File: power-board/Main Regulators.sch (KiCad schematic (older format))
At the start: 19 parts, among them U201 LMZ23610

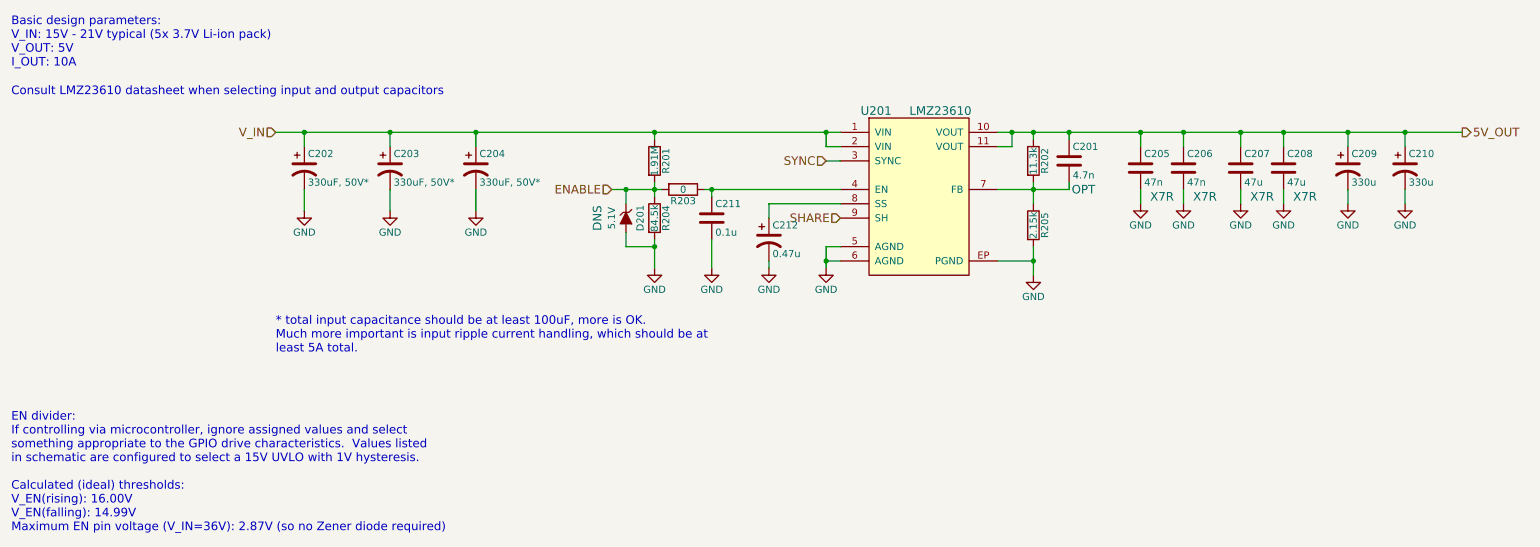
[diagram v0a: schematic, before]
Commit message: routed board
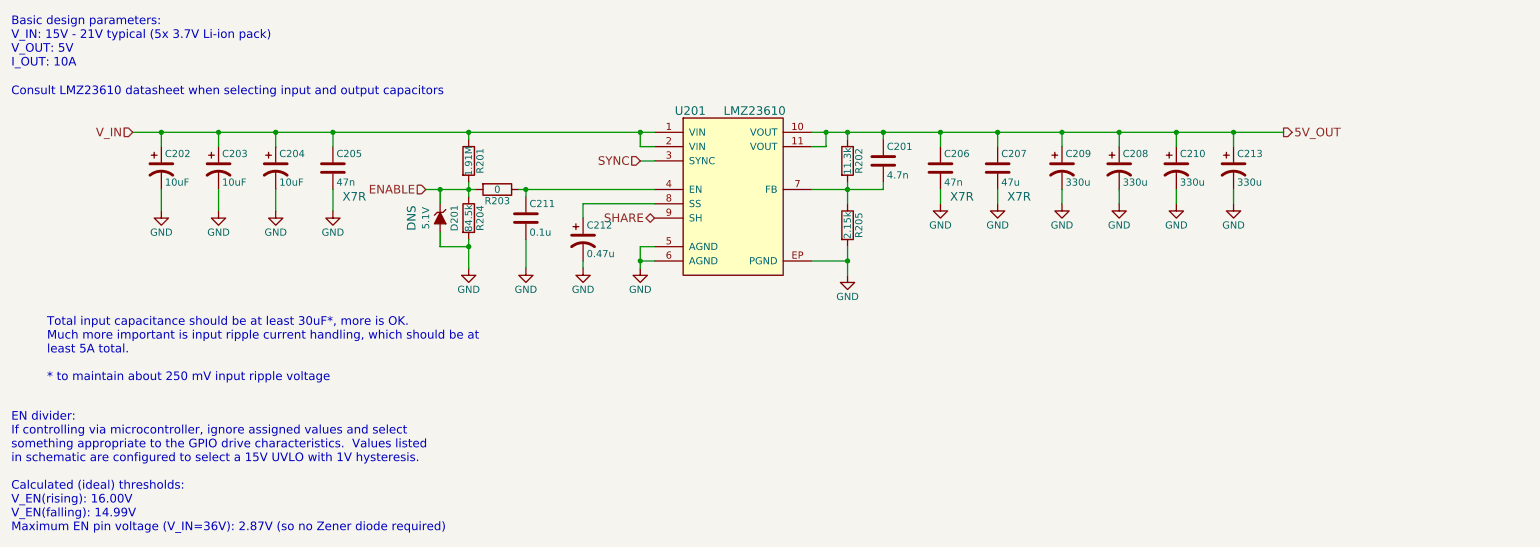
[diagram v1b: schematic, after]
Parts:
- removed C208: 47u, symbol C
- added C208, C213: 330u, Capacitors_Tantalum_SMD:Tantalum_Case-V_EIA-7343-20_Hand, symbol CP1
- C201: footprint (none) -> Capacitors_SMD:C_0603; MFG (none) -> Samsung; MPN (none) -> CL10B472KB8NNNC; Note OPT -> (none)
- C202, C203, C204: value 330uF, 50V* -> 10uF; footprint (none) -> Capacitors_SMD:C_1210; MFG Panasonic Electronic Components -> TDK Corporation; MPN EEU-FM1H331L -> C3225X7S1H106M250AB; Note (none) -> 50V, Low ESL
- C205, C206, C211, C212: footprint (none) -> Capacitors_SMD:C_0603
- C207: footprint (none) -> Capacitors_SMD:C_0805
- C209, C210: footprint (none) -> Capacitors_Tantalum_SMD:Tantalum_Case-V_EIA-7343-20_Hand; MFG Kemet -> AVX Corporation; MPN A750KK337M1CAAE014 -> TCJD337M006R0025; Note low-ESR -> 6.3V, 0.025 ohm
- D201: footprint (none) -> Diodes_SMD:D_SOD-123
- R201: footprint (none) -> Resistors_SMD:R_0805; MFG Vishay -> Yageo; MPN CRCW06031M91FKEA -> RC0805FR-071M91L
- R202: footprint (none) -> Resistors_SMD:R_0805; MFG Vishay -> Yageo; MPN CRCW060311K3FKEA -> RC0805FR-0711K3L
- R203: footprint (none) -> Resistors_SMD:R_0805
- R204: footprint (none) -> Resistors_SMD:R_0805; MFG Vishay -> Yageo; MPN CRCW060384K5FKEA -> RC0805FR-0784K5L
- R205: footprint (none) -> Resistors_SMD:R_0805; MFG (none) -> Yageo; MPN (none) -> RC0805FR-072K15L
- U201: footprint (none) -> project:TO-PMOD-11
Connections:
- net 5V_OUT: now also C208.1, C213.1; no longer C205.1
- net GND: now also C208.2, C213.2
- net V_IN: now also C205.1
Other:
- note added: "Total input capacitance should be at least 30uF*, more is OK.\nMuch more important is input ripple current handling, which should be at\nleast 5A total.\n\n* to maintain about 250 mV input ripple voltage"
- note removed: "* total input capacitance should be at least 100uF, more is OK.\nMuch more important is input ripple current handling, which should be at\nleast 5A total."
- moved on the sheet: C202, C205, C206, C207, C209, C211, C212, D201, R201, R202, R203, R204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
